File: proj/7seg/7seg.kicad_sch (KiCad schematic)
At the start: 22 parts, among them J1 Conn_01x05_Pin, U1 74HC595, U2 74HC595

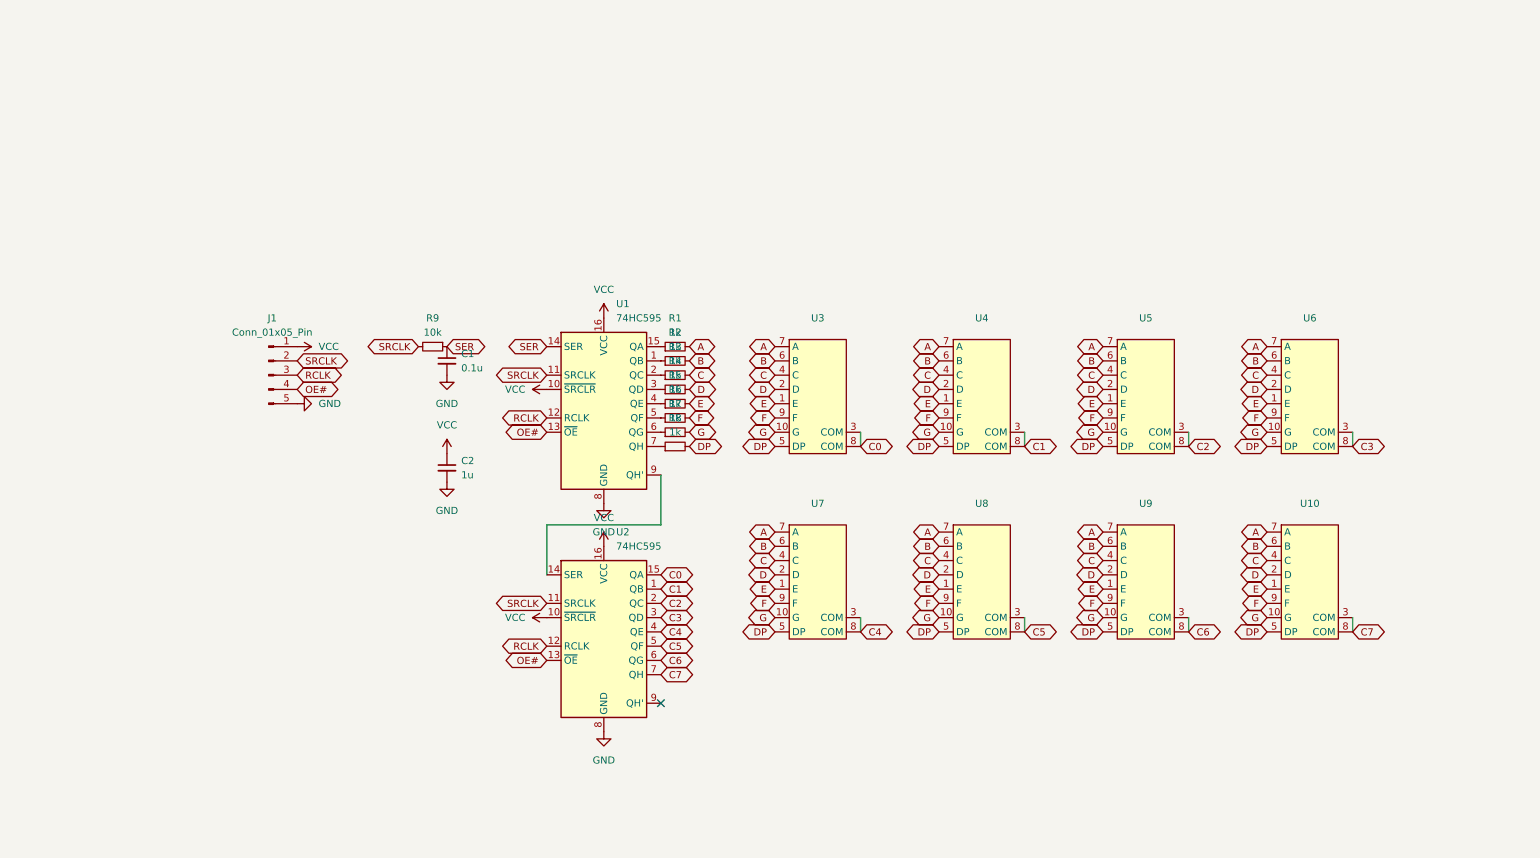
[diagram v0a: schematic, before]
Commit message: -
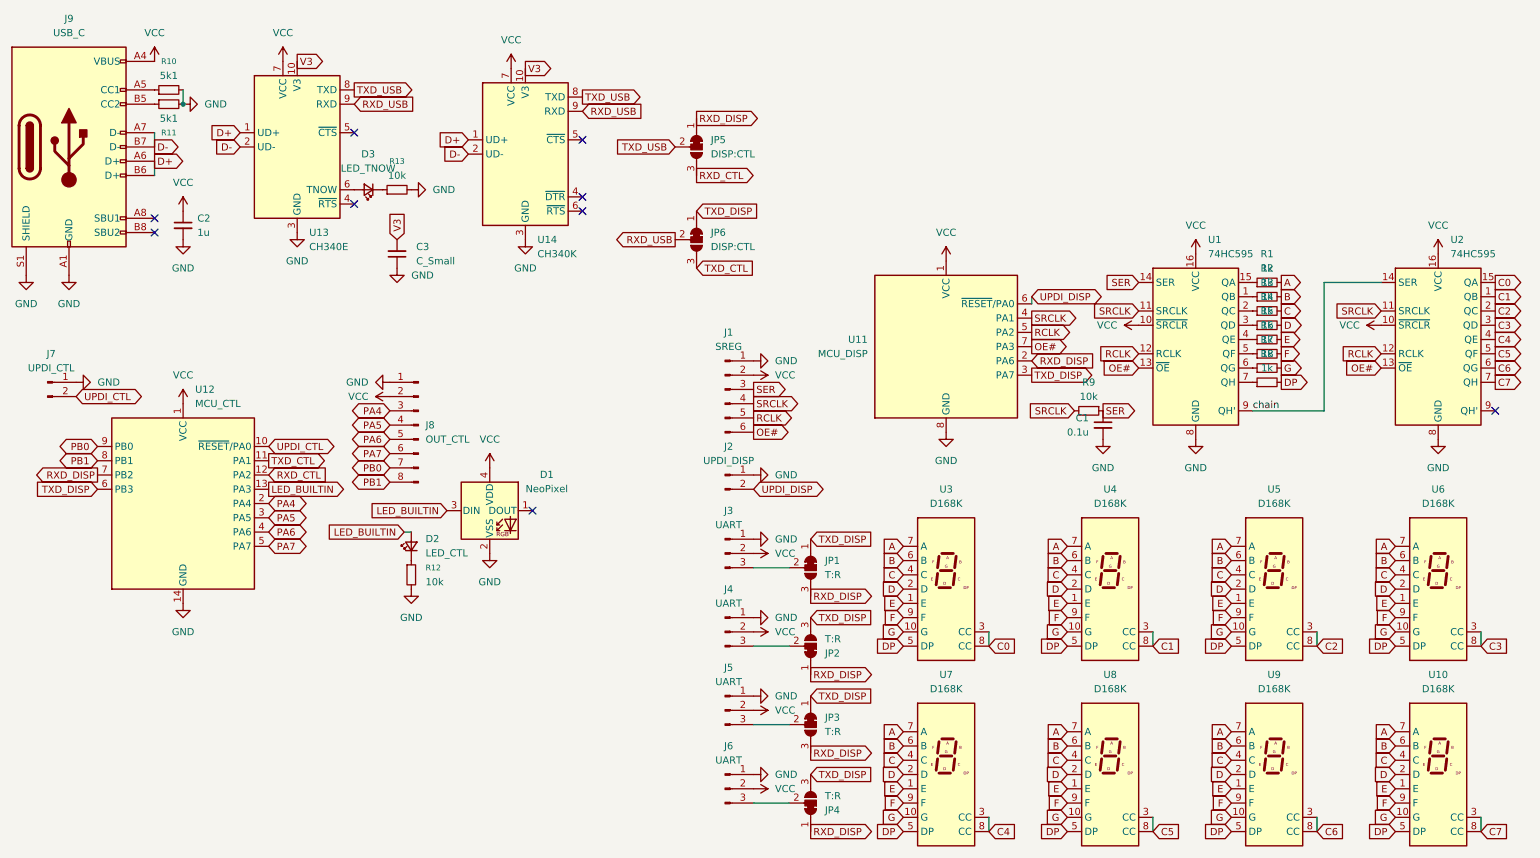
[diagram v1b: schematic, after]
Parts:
- removed J1: Conn_01x05_Pin, Connector_PinHeader_2.54mm:PinHeader_1x05_P2.54mm_Vertical, symbol Connector:Conn_01x05_Pin
- removed U10, U3, U4, U5, U6, U7, U8, U9: ~, Library:LA-501DD, symbol Library:LA-501DD
- added C3: C_Small, symbol Device:C_Small
- added D1: NeoPixel, LED_SMD:LED_WS2812B-2020_PLCC4_2.0x2.0mm, symbol LED:WS2812B-2020
- added D2: LED_CTL, symbol Device:LED_Small
- added D3: LED_TNOW, symbol Device:LED_Small
- added J1: SREG, Connector_PinHeader_2.54mm:PinHeader_1x03_P2.54mm_Vertical, symbol Connector:Conn_01x06_Pin
- added J2: UPDI_DISP, Connector_PinHeader_2.54mm:PinHeader_1x02_P2.54mm_Vertical, symbol Connector:Conn_01x02_Pin
- added J3, J4, J5, J6: UART, Connector_PinHeader_2.54mm:PinHeader_1x03_P2.54mm_Vertical, symbol Connector:Conn_01x03_Pin
- added J7: UPDI_CTL, Connector_PinHeader_2.54mm:PinHeader_1x02_P2.54mm_Vertical, symbol Connector:Conn_01x02_Pin
- added J8: OUT_CTL, symbol Connector:Conn_01x08_Pin
- added J9: USB_C, symbol Connector:USB_C_Receptacle_USB2.0_16P
- added JP1, JP2, JP3, JP4: T:R, Jumper:SolderJumper-3_P1.3mm_Bridged12_RoundedPad1.0x1.5mm, symbol Jumper:SolderJumper_3_Bridged12
- added JP5, JP6: DISP:CTL, Jumper:SolderJumper-3_P1.3mm_Bridged12_RoundedPad1.0x1.5mm, symbol Jumper:SolderJumper_3_Bridged12
- added R10, R11: 5k1, Resistor_SMD:R_0603_1608Metric, symbol Device:R_Small
- added R12, R13: 10k, symbol Device:R_Small
- added U10, U3, U4, U5, U6, U7, U8, U9: D168K, Display_7Segment:D1X8K, symbol Display_Character:D168K
- added U11: MCU_DISP, Package_SO:SOIC-8_3.9x4.9mm_P1.27mm, symbol MCU_Microchip_ATtiny:ATtiny402-SS
- added U12: MCU_CTL, Package_SO:SOIC-14_3.9x8.7mm_P1.27mm, symbol MCU_Microchip_ATtiny:ATtiny1604-SS
- added U13: CH340E, Package_SO:MSOP-10_3x3mm_P0.5mm, symbol Interface_USB:CH340E
- added U14: CH340K, Package_SO:SSOP-10-1EP_3.9x4.9mm_P1mm_EP2.1x3.3mm, symbol Interface_USB:CH340K
- U1, U2: footprint Package_SO:SOP-16_4.55x10.3mm_P1.27mm -> Package_SO:TSSOP-16_4.4x5mm_P0.65mm
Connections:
- net A: now also U10.7 (A), U3.7 (A), U4.7 (A), U5.7 (A), U6.7 (A), U7.7 (A), U8.7 (A), U9.7 (A)
- net B: now also U10.6 (B), U3.6 (B), U4.6 (B), U5.6 (B), U6.6 (B), U7.6 (B), U8.6 (B), U9.6 (B)
- net C: now also U10.4 (C), U3.4 (C), U4.4 (C), U5.4 (C), U6.4 (C), U7.4 (C), U8.4 (C), U9.4 (C)
- net C0: now also U3.3 (CC), U3.8 (CC)
- net C1: now also U4.3 (CC), U4.8 (CC)
- net C2: now also U5.3 (CC), U5.8 (CC)
- net C3: now also U6.3 (CC), U6.8 (CC)
- net C4: now also U7.3 (CC), U7.8 (CC)
- net C5: now also U8.3 (CC), U8.8 (CC)
- net C6: now also U9.3 (CC), U9.8 (CC)
- net C7: now also U10.3 (CC), U10.8 (CC)
- net D: now also U10.2 (D), U3.2 (D), U4.2 (D), U5.2 (D), U6.2 (D), U7.2 (D), U8.2 (D), U9.2 (D)
- net DP: now also U10.5 (DP), U3.5 (DP), U4.5 (DP), U5.5 (DP), U6.5 (DP), U7.5 (DP), U8.5 (DP), U9.5 (DP)
- net E: now also U10.1 (E), U3.1 (E), U4.1 (E), U5.1 (E), U6.1 (E), U7.1 (E), U8.1 (E), U9.1 (E)
- net F: now also U10.9 (F), U3.9 (F), U4.9 (F), U5.9 (F), U6.9 (F), U7.9 (F), U8.9 (F), U9.9 (F)
- net G: now also U10.10 (G), U3.10 (G), U4.10 (G), U5.10 (G), U6.10 (G), U7.10 (G), U8.10 (G), U9.10 (G)
- net GND: now also C3.1, D1.2 (VSS), J1.1 (Pin_1), J2.1 (Pin_1), J3.1 (Pin_1), J4.1 (Pin_1), J5.1 (Pin_1), J6.1 (Pin_1), J7.1 (Pin_1), J8.1 (Pin_1), J9.A1 (GND), J9.A12 (GND), J9.B1 (GND), J9.B12 (GND), J9.S1 (SHIELD), R10.2, R11.2, R12.2, R13.2, U11.8 (GND), U12.14 (GND), U13.3 (GND), U14.11 (GND), U14.3 (GND)
- net OE#: now also J1.6 (Pin_6), U11.7 (PA3)
- net RCLK: now also J1.5 (Pin_5), U11.5 (PA2)
- net SER: now also J1.3 (Pin_3)
- net SRCLK: now also J1.4 (Pin_4), U11.4 (PA1)
- net VCC: now also D1.4 (VDD), J1.2 (Pin_2), J3.2 (Pin_2), J4.2 (Pin_2), J5.2 (Pin_2), J6.2 (Pin_2), J8.2 (Pin_2), J9.A4 (VBUS), J9.A9 (VBUS), J9.B4 (VBUS), J9.B9 (VBUS), U11.1 (VCC), U12.1 (VCC), U13.7 (VCC), U14.7 (VCC)
- net chain: now reaches U1.9 (QH'), U2.14 (SER)
- new net: J9.A5 (CC1), R10.1
- new net: D3.1 (K), R13.1
- new net: D3.2 (A), U13.6 (TNOW)
- new net: J6.3 (Pin_3), JP4.2 (C)
- new net: D2.1 (K), R12.1
- new net: J4.3 (Pin_3), JP2.2 (C)
- new net: J3.3 (Pin_3), JP1.2 (C)
- new net: J5.3 (Pin_3), JP3.2 (C)
- new net: J9.B5 (CC2), R11.1
- new net D+: J9.A6 (D+), J9.B6 (D+), U13.1 (UD+), U14.1 (UD+)
- new net D-: J9.A7 (D-), J9.B7 (D-), U13.2 (UD-), U14.2 (UD-)
- new net LED_BUILTIN: D1.3 (DIN), D2.2 (A), U12.13 (PA3)
- new net PA4: J8.3 (Pin_3), U12.2 (PA4)
- new net PA5: J8.4 (Pin_4), U12.3 (PA5)
- new net PA6: J8.5 (Pin_5), U12.4 (PA6)
- new net PA7: J8.6 (Pin_6), U12.5 (PA7)
- new net PB0: J8.7 (Pin_7), U12.9 (PB0)
- new net PB1: J8.8 (Pin_8), U12.8 (PB1)
- new net RXD_CTL: JP5.3 (B), U12.12 (PA2)
- new net RXD_DISP: JP1.3 (B), JP2.1 (A), JP3.3 (B), JP4.1 (A), JP5.1 (A), U11.2 (PA6), U12.7 (PB2)
- new net RXD_USB: JP6.2 (C), U13.9 (RXD), U14.9 (RXD)
- new net TXD_CTL: JP6.3 (B), U12.11 (PA1)
- new net TXD_DISP: JP1.1 (A), JP2.3 (B), JP3.1 (A), JP4.3 (B), JP6.1 (A), U11.3 (PA7), U12.6 (PB3)
- new net TXD_USB: JP5.2 (C), U13.8 (TXD), U14.8 (TXD)
- new net UPDI_CTL: J7.2 (Pin_2), U12.10 (~{RESET}/PA0)
- new net UPDI_DISP: J2.2 (Pin_2), U11.6 (~{RESET}/PA0)
- new net V3: C3.2, U13.10 (V3), U14.10 (V3)
- no-connect marks 1 -> 9
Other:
- moved on the sheet: C1, C2, R1, R2, R3, R4, R5, R6, R7, R8, R9, U1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
